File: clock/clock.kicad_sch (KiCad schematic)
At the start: 29 parts, among them J1 Conn_01x06, J2 PJ-102AH, SW1 Omron_B3F_SPST, U1 ATmega328-PU, U2 L7805, U3 MAX7219, Y1 Crystal_16MHz

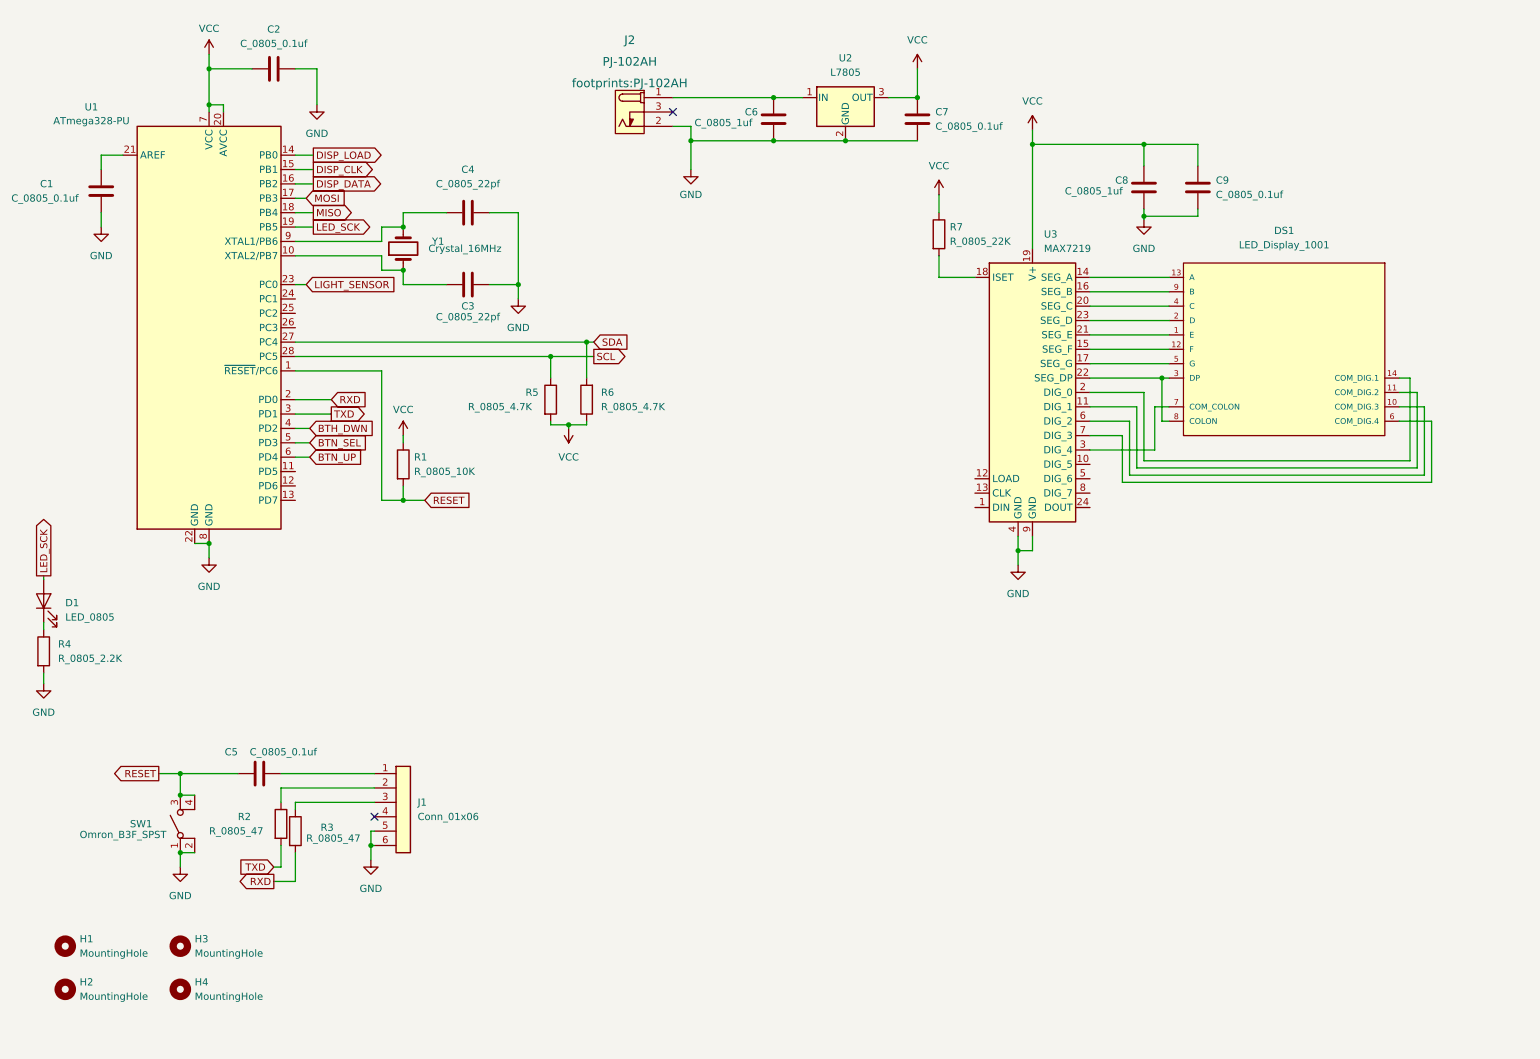
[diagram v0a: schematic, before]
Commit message: pre review schematic
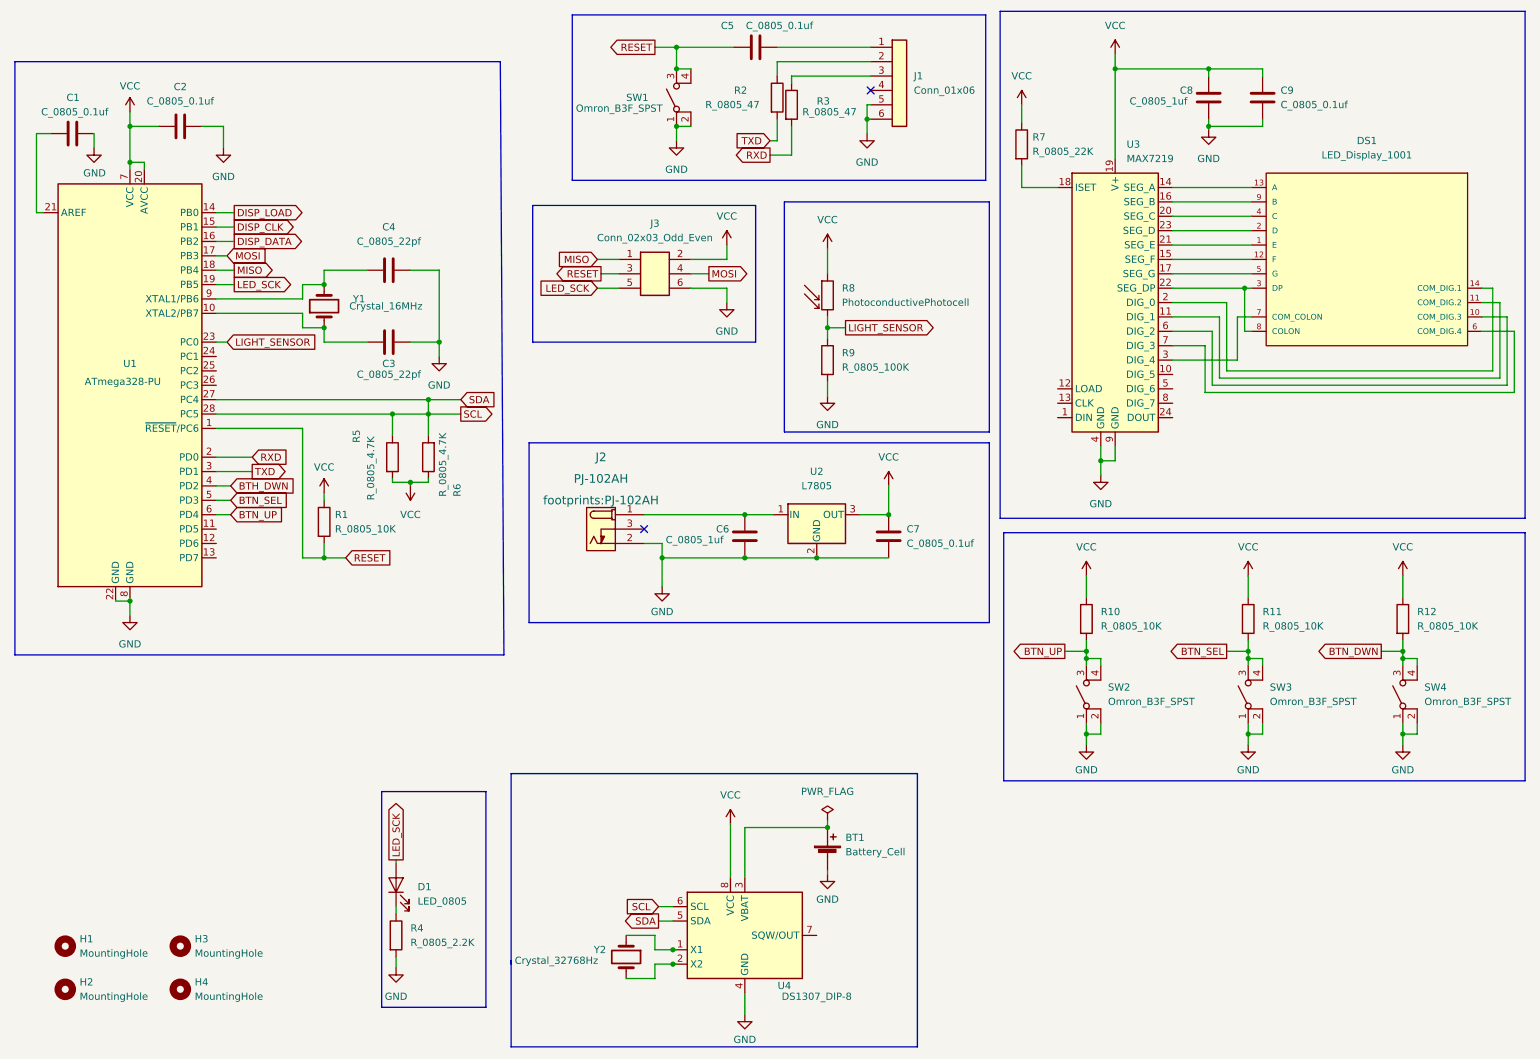
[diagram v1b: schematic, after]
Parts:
- added BT1: Battery_Cell, footprints:BatteryHolder_Keystone_106_1x20mm, symbol HPS:Battery_Cell
- added J3: Conn_02x03_Odd_Even, footprints:PinHeader_2x03_P2.54mm_Vertical, symbol HPS:Conn_02x03_Odd_Even
- added R10, R11, R12: R_0805_10K, footprints:R_0805_2012Metric, symbol HPS:R_0805_10K
- added R8: PhotoconductivePhotocell, footprints:R_LDR_4.9x4.2mm_P2.54mm_Vertical, symbol HPS:PhotoconductivePhotocell
- added R9: R_0805_100K, footprints:R_0805_2012Metric, symbol HPS:R_0805_100K
- added SW2, SW3, SW4: Omron_B3F_SPST, footprints:SW_SPST_Omron_B3FS-100xP, symbol HPS:Omron_B3F_SPST
- added U4: DS1307_DIP-8, footprints:DIP-8_W7.62mm, symbol HPS:DS1307_DIP-8
- added Y2: Crystal_32768Hz, footprints:Crystal_SMD_2Pin_3.2x1.5mm, symbol HPS:Crystal_32768Hz
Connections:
- net SDA is gone; now on net SCL: R6.2, U1.27 (PC4)
- net BTN_SEL: now also R11.2, SW3.3 (B), SW3.4 (B)
- net BTN_UP: now also R10.2, SW2.3 (B), SW2.4 (B)
- net GND: now also BT1.2 (-), J3.6 (Pin_6), R9.2, SW2.1 (A), SW2.2 (A), SW3.1 (A), SW3.2 (A), SW4.1 (A), SW4.2 (A), U4.4 (GND)
- net LED_SCK: now also J3.5 (Pin_5)
- net LIGHT_SENSOR: now also R8.2, R9.1
- net MISO: now also J3.1 (Pin_1)
- net MOSI: now also J3.4 (Pin_4)
- net RESET: now also J3.3 (Pin_3)
- net SCL: now also U4.5 (SDA), U4.6 (SCL)
- net VCC: now also J3.2 (Pin_2), R10.1, R11.1, R12.1, R8.1, U4.8 (VCC)
- new net: U4.1 (X1), Y2.1
- new net: U4.2 (X2), Y2.2
- new net: BT1.1 (+), U4.3 (VBAT)
- new net BTN_DWN: R12.2, SW4.3 (B), SW4.4 (B)
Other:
- moved on the sheet: C1, C2, C3, C4, C5, C6, C7, C8, C9, D1, DS1, J1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
